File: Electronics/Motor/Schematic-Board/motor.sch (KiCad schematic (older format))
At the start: 42 parts, among them J1 CONN_02X05, J11 V, J12 U, J13 W, J2 RS485, J3 RS485, J4 CONN_01X06, J5 JTAG, J6 12, J9 GND, Q1 PSMN3R3-40YS, Q2 PSMN3R3-40YS, Q3 PSMN3R3-40YS, Q4 PSMN3R3-40YS, Q5 PSMN3R3-40YS, Q6 PSMN3R3-40YS, U1 STSPIN32F0, U2 LTC2876, U3 MA700, Y1 8Mhz

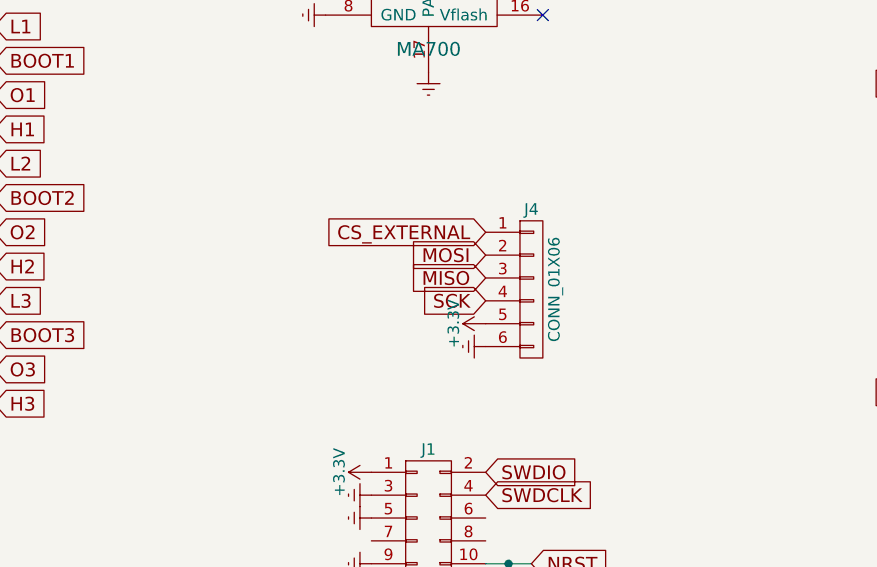
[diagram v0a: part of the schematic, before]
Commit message: current work
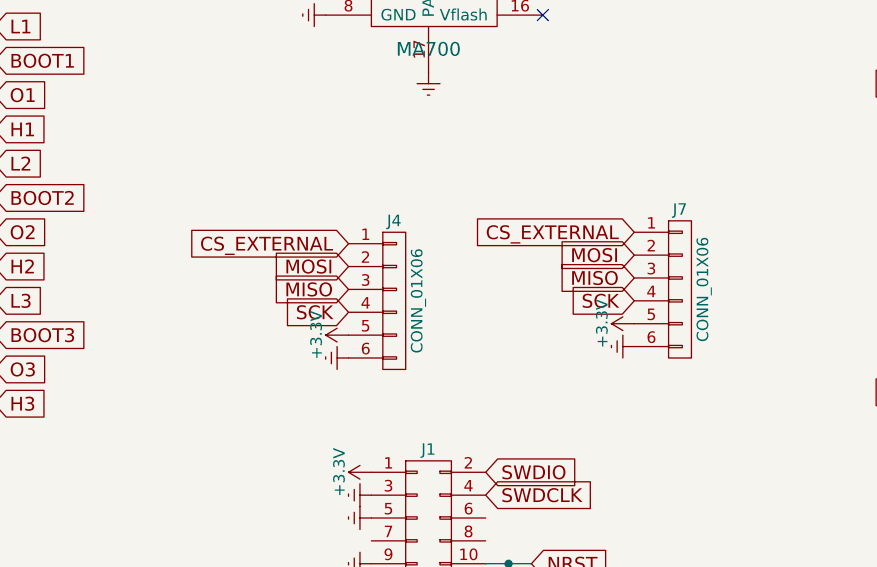
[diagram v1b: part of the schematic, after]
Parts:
- added J7: CONN_01X06, Dizzy:SPI_CONN, symbol CONN_01X06
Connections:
- net +3V3: now also J7.5 (P5)
- net CS_EXTERNAL: now also J7.1 (P1)
- net Earth: now also J7.6 (P6)
- net MISO: now also J7.3 (P3)
- net MOSI: now also J7.2 (P2)
- net SCK: now also J7.4 (P4)
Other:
- moved on the sheet: J4

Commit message: saving changes
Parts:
- D5: footprint LEDs:LED_0603 -> LEDs:LED_0805_HandSoldering
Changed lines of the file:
@@
 F 0 "D5" H 2150 4450 50  0000 C CNN
 F 1 "STATUS" H 2150 4250 50  0000 C CNN
-F 2 "LEDs:LED_0603" H 2150 4350 50  0001 C CNN
+F 2 "LEDs:LED_0805_HandSoldering" H 2150 4350 50  0001 C CNN
 F 3 "" H 2150 4350 50  0001 C CNN
 	1    2150 4350
